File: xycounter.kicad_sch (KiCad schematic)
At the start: 18 parts, among them J10 PosResets, J11 Power and Clock, J8 posX, J9 posY, U1 74LS163, U10 74LS30, U110 74LS08, U111 74LS30, U19 74LS32, U2 74LS163, U3 74LS163, U4 74LS163, U5 74LS163, U6 74LS163, U69 74LS30, U7 74LS30, U8 74LS04, U9 74LS32

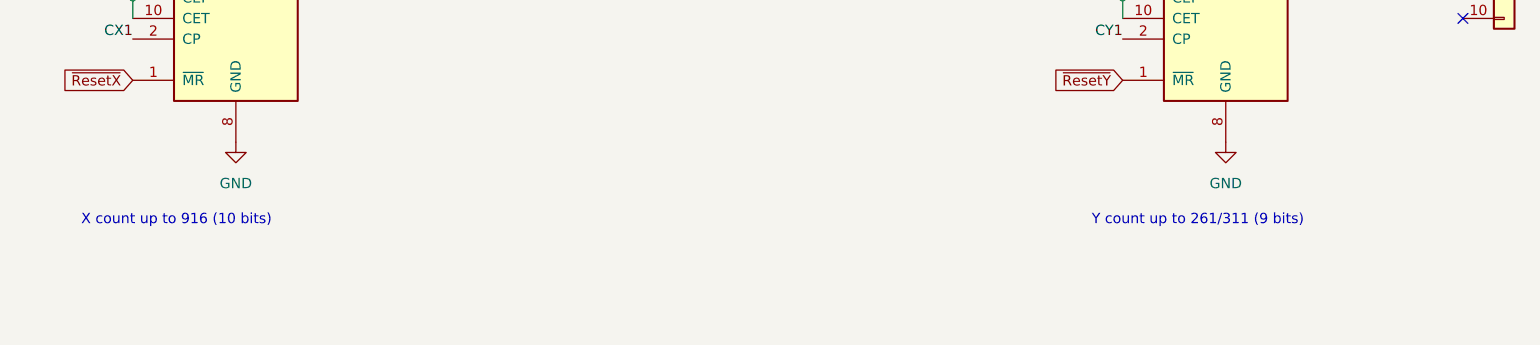
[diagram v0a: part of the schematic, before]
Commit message: refine main board layout
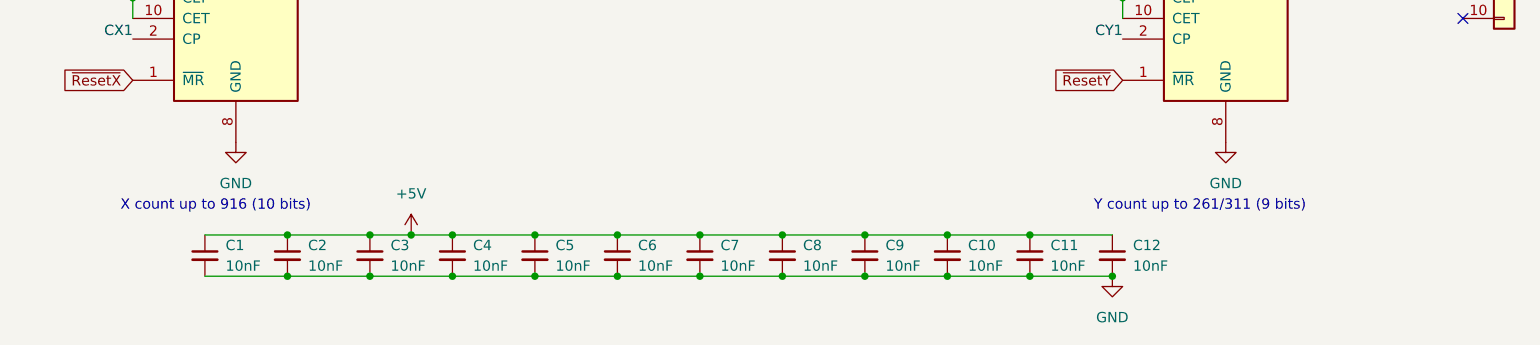
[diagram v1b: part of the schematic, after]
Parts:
- added C1, C10, C11, C12, C2, C3, C4, C5, C6, C7, C8, C9: 10nF, Capacitor_SMD:C_0603_1608Metric, symbol Device:C_Small
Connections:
- net +5V: now also C1.1, C10.1, C11.1, C12.1, C2.1, C3.1, C4.1, C5.1, C6.1, C7.1, C8.1, C9.1
- net GND: now also C1.2, C10.2, C11.2, C12.2, C2.2, C3.2, C4.2, C5.2, C6.2, C7.2, C8.2, C9.2
